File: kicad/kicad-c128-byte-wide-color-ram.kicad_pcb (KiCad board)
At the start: 2 copper layers, 22.9 x 51.3 mm, 7 parts, among them J1 A11_A14, J2 AEC, J3 D4_D7, U1 2016-board, U2 KM62256CLP, U3 2016, U4 4066

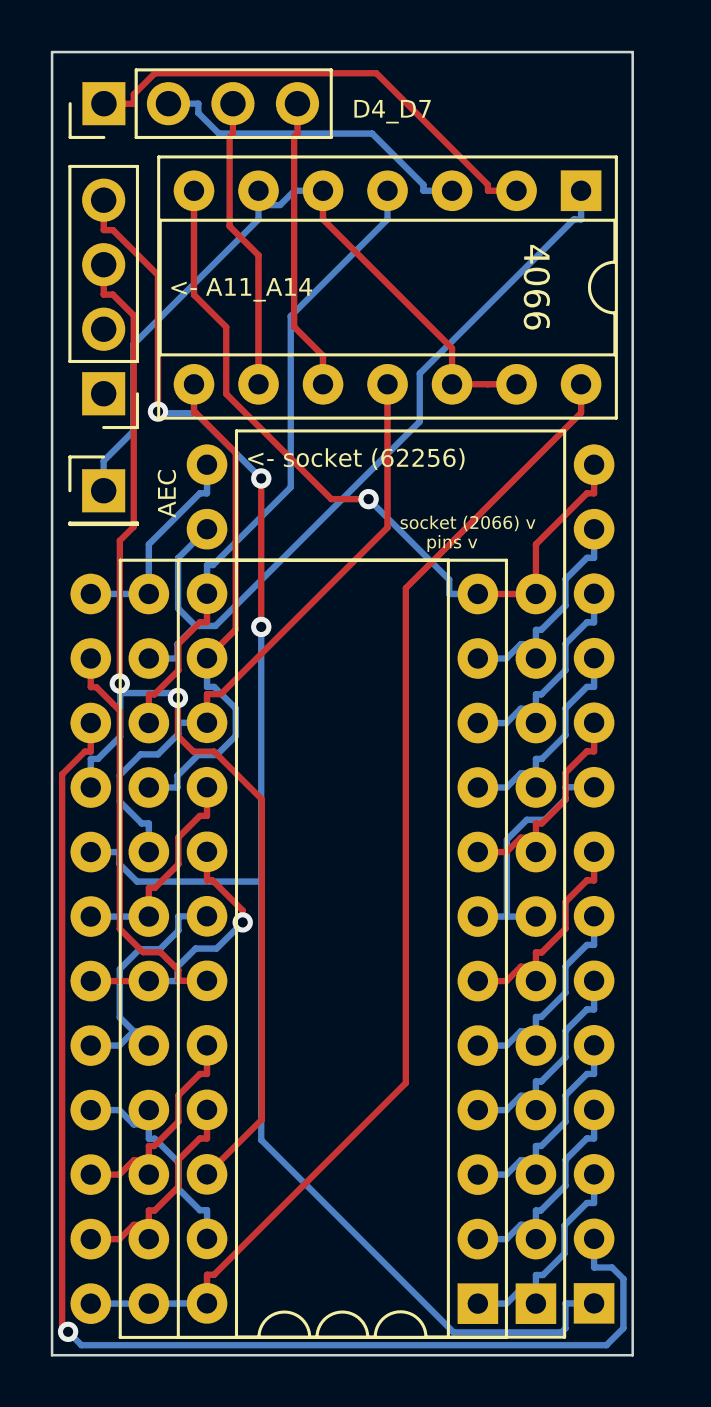
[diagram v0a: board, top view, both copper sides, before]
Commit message: revision 1.1 with 1571CR info
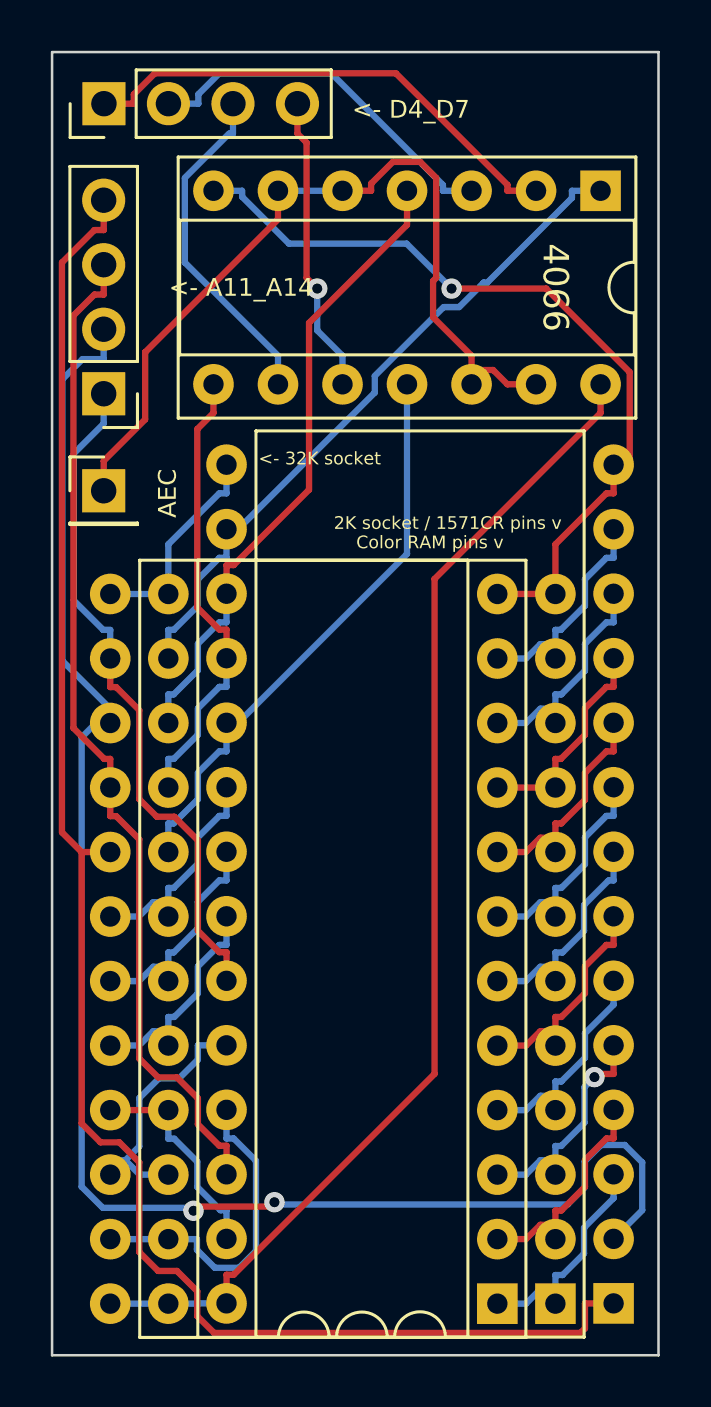
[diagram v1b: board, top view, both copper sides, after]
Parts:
- J3: value D4_D7 -> <- D4_D7
- moved U1 0.77 mm to (122.4, 112.3)
- moved U2 0.77 mm to (127.0, 112.3)
- moved U3 0.77 mm to (124.7, 112.3)
- moved U4 0.77 mm to (126.5, 68.5)
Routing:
- net /A12: track 51.4 -> 64.7 mm, vias 1 -> 2
- net /A11: track 15.8 -> 27.0 mm
- net /A13: track 46.0 -> 39.9 mm, vias 2 -> 0
- net /A8: track 8.86 -> 12.9 mm
- net /D4: track 31.3 -> 27.3 mm
- net /AEC: track 29.4 -> 33.4 mm
- net /D6: track 20.2 -> 18.0 mm
- net GND: track 30.5 -> 32.4 mm
- net /A10: track 10.8 -> 8.85 mm, vias 1 -> 0
- net /D6_bus: track 11.6 -> 13.4 mm
- net /D5_bus: track 12.9 -> 14.7 mm
- net /D7: track 24.8 -> 23.1 mm
- net /A9: track 8.85 -> 10.4 mm
- net /~{OE}: track 10.4 -> 8.86 mm
- net /A14: track 65.4 -> 66.8 mm, vias 3 -> 0
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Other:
- board size 22.9 x 51.3 mm -> 23.9 x 51.3 mm
- board text added: "2K socket / 1571CR pins v"
- board text added: "<- 32K socket"
- board text added: "C128 bytewide 2/32K Color RAM v1.1 C128DCR / 157CR RAM expansion v1.1 Maciej Witkowiak <ytm@elysium.pl>, XI 2023"
- board text added: "Color RAM pins v"
- board text removed: "<- socket (62256)"
- board text removed: "C128 bytewide 2/32K Color RAM v1.0 Maciej Witkowiak <ytm@elysium.pl>, X 2023"
- board text removed: "pins v"
- board text removed: "socket (2066) v"
